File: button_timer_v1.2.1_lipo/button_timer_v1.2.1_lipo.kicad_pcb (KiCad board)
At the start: 2 copper layers, 21 x 41.7 mm, 22 parts, among them J1 Conn_01x05_Female, SW1 SW_Push, SW2 SW_Push, U2 AP2112K-3.3, U3 TPL5111, X1 ESP-12E

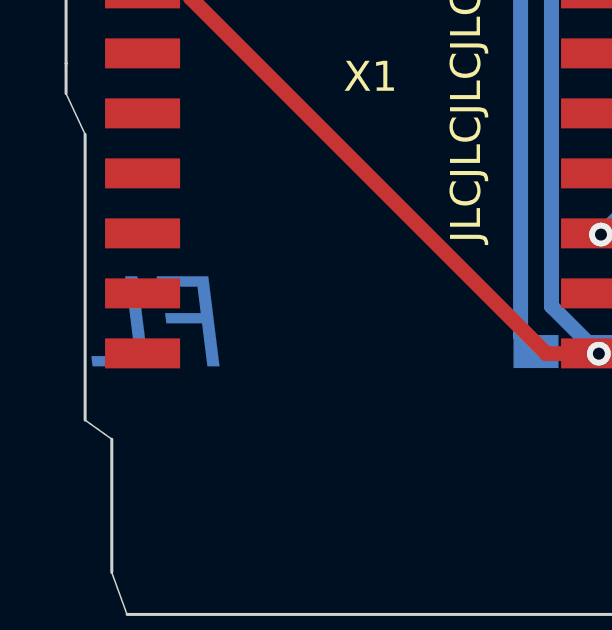
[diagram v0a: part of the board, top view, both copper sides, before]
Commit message: 23.02 00:38
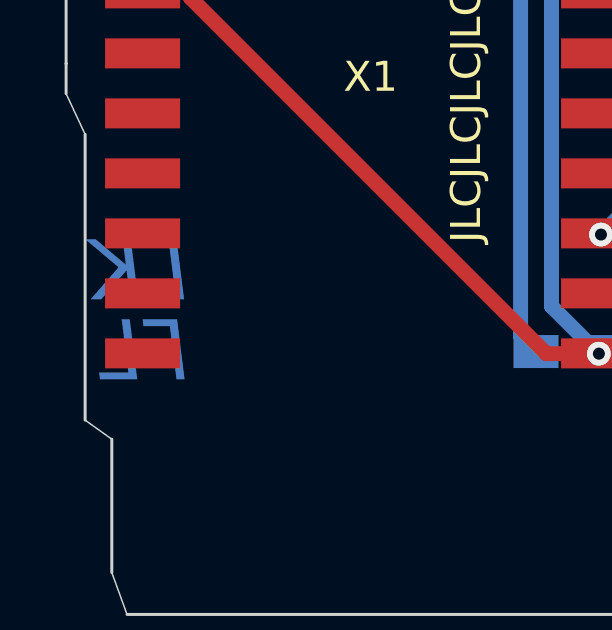
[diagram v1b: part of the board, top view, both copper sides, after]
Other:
- board text added: "LK"
